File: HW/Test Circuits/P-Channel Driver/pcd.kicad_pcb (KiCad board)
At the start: 2 copper layers, 15 parts, among them J1 PWR, J2 PWM_IN, J3 OUT, Q1 BC546B, Q2 BC546B, Q3 IRF9530

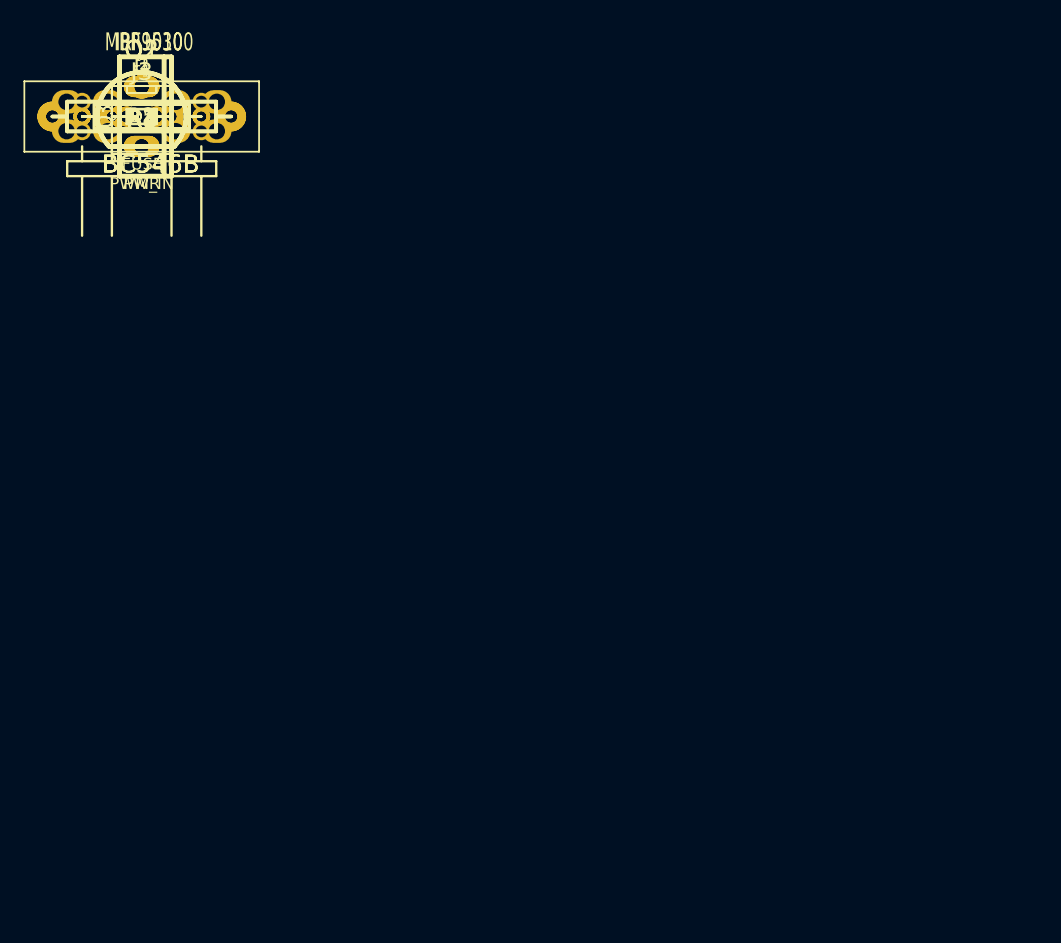
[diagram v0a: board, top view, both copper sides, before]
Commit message: The first wave of test boards finished
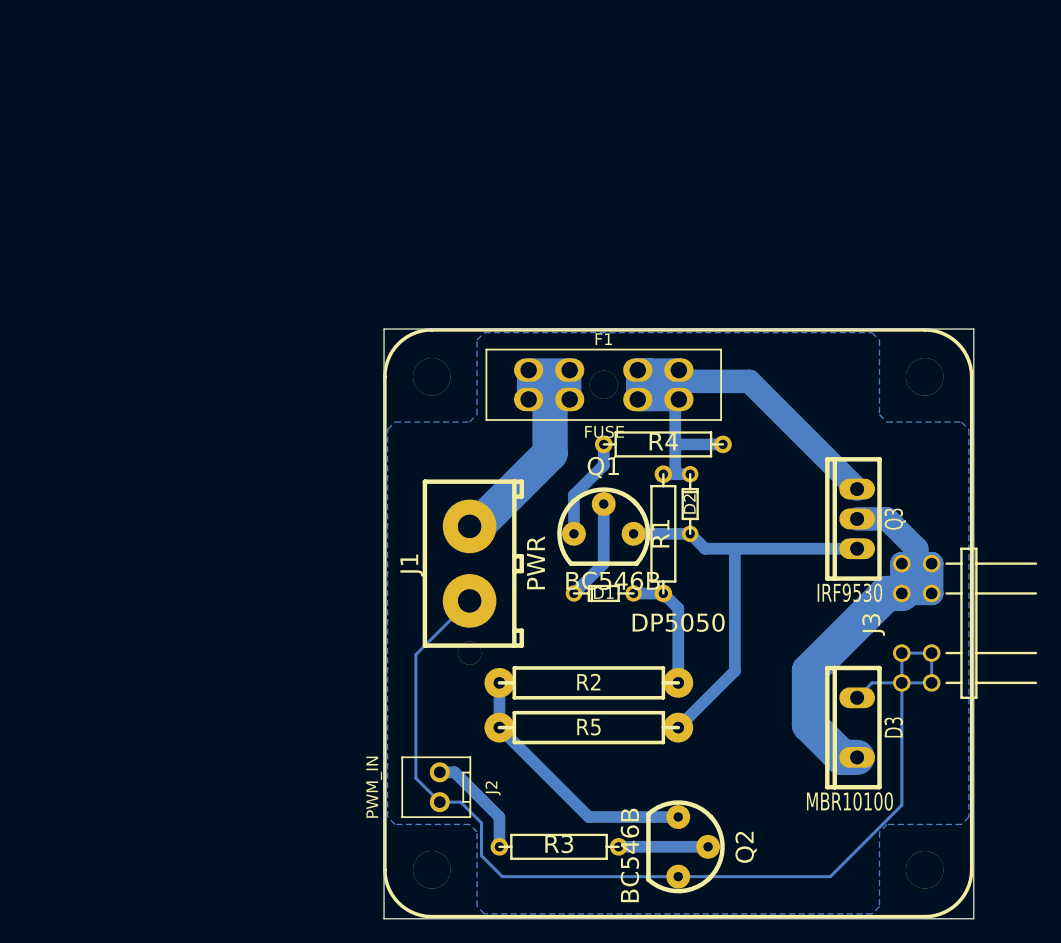
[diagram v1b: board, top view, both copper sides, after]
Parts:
- added DP5050: , DP5050, F.Cu at (45.7, 43.2)
- J1: footprint CONN_NCW254-02S -> MOLEX_36538_2
- moved D3 80.2 mm to (61.0, 52.1), turned to 180 degrees
- moved J3 78.9 mm to (66.0, 43.2), turned to 90 degrees
- moved Q2 77.2 mm to (45.7, 62.2), turned to 270 degrees
- moved R3 71.7 mm to (35.6, 62.2), turned to 180 degrees
- moved Q3 69.9 mm to (61.0, 34.3), turned to 180 degrees
- moved R5 64.5 mm to (38.1, 52.1)
- moved J2 62.5 mm to (25.4, 57.1), turned to 270 degrees
- moved R2 61.5 mm to (38.1, 48.3)
- moved D2 57.2 mm to (46.7, 33.0), turned to 90 degrees
- moved R1 56.9 mm to (44.5, 35.6), turned to 270 degrees
- moved D1 56.6 mm to (39.4, 40.6), turned to 180 degrees
- moved Q1 53.1 mm to (39.4, 35.6)
- moved R4 52.5 mm to (44.5, 27.9), turned to 180 degrees
- moved J1 47.2 mm to (27.9, 38.1), turned to 90 degrees
- moved F1 45.5 mm to (39.4, 22.9)
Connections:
- D2 pad 2: N-000006 (its old number) -> N-000005
- F1 pad 2: N-000006 (its old number) -> N-000005
- J1 pad 1: VDD -> GND
- J1 pad 2: GND -> VDD
- Q3 pad 3: N-000006 (its old number) -> N-000005
- R1 pad 1: VDD -> N-000005
- R4 pad 1: N-000006 (its old number) -> N-000005
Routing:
- net GND: track 0.00 -> 91.0 mm
- net N-000005: track 0.00 -> 54.4 mm
- net N-000006: track 0.00 -> 44.6 mm
- net N-000008: track 0.00 -> 36.8 mm
- net VDD: track 0.00 -> 27.0 mm
- net N-000004: track 0.00 -> 22.2 mm
- net N-000009: track 0.00 -> 10.7 mm
- net N-000002: track 0.00 -> 9.20 mm
- net N-0000011: track 0.00 -> 8.67 mm
- net N-0000010: track 0.00 -> 8.67 mm
- net N-000007: track 0.00 -> 7.62 mm
- added copper zone on B.Cu, net GND
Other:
- board outline added: 50.3 x 50.2 mm
